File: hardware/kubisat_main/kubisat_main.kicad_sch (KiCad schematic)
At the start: 51 parts, among them J1 DEBUG_SWD, J2 Micro_SD_Card_Det1, J3 UART0, J4 POWER_IN, J5 IPX, Q1 BSS138, Q2 BSS138, SW1 BOOTSEL, SW2 RESET, U1 W25Q16JVSS, U2 RP2040, U3 NEO-6M-GPS, U4 XL1278-SMT, Y1 12MHz

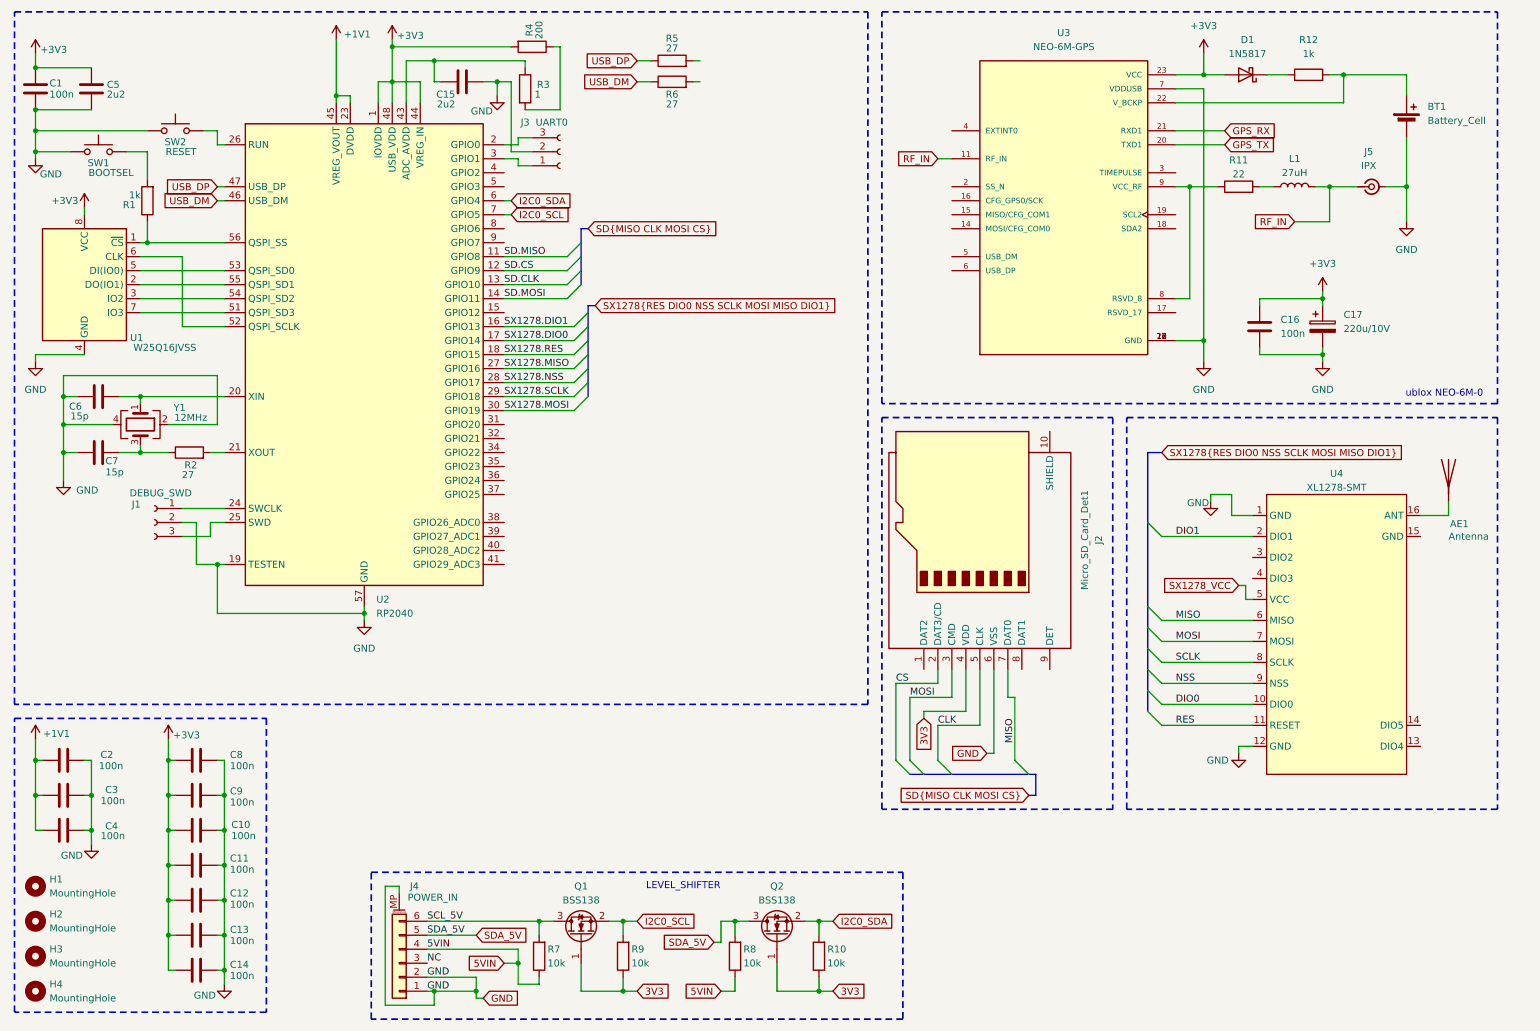
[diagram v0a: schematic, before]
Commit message: completed (?) mainboard schematic
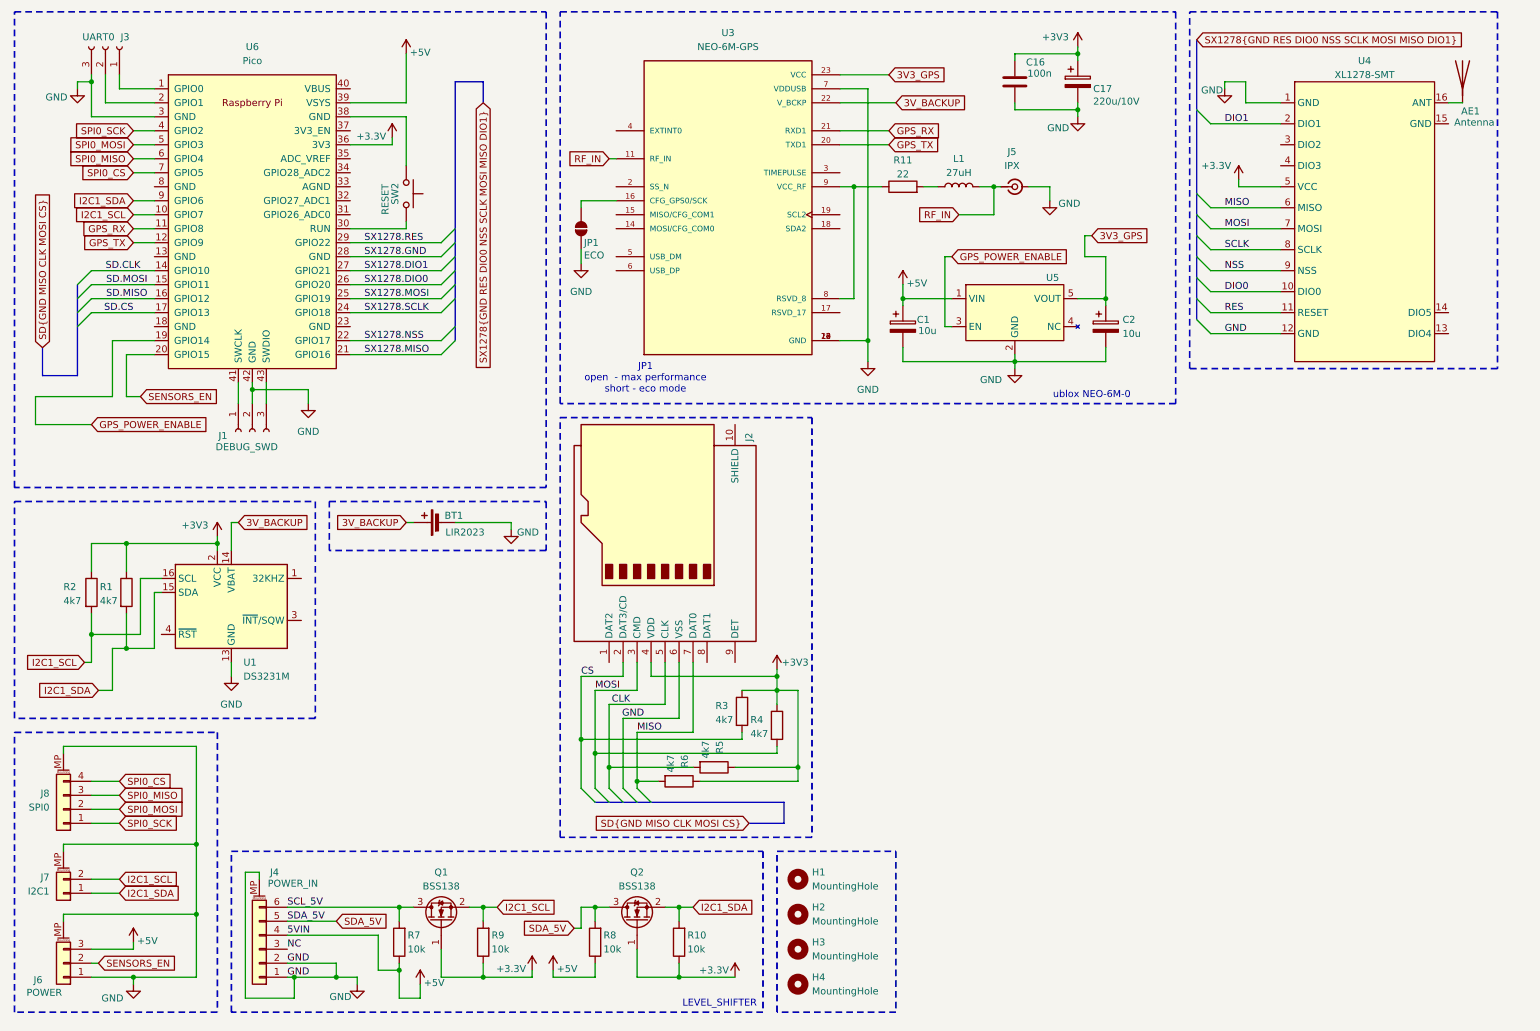
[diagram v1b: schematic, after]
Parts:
- removed C1, C10, C11, C12, C13, C14, C2, C3, C4, C8, C9: 100n, Capacitor_SMD:C_0805_2012Metric, symbol Device:C
- removed C15, C5: 2u2, Capacitor_SMD:C_0805_2012Metric, symbol Device:C
- removed C6, C7: 15p, Capacitor_SMD:C_0805_2012Metric, symbol Device:C
- removed D1: 1N5817, Diode_SMD:D_SOD-123, symbol Device:D_Schottky
- removed R12: 1k, Resistor_SMD:R_0805_2012Metric, symbol Device:R
- removed SW1: BOOTSEL, Button_Switch_SMD:SW_MEC_5GSH9, symbol Switch:SW_Push
- removed U1: W25Q16JVSS, Package_SO:SOIC-8_5.23x5.23mm_P1.27mm, symbol Memory_Flash:W25Q16JVSS
- removed U2: RP2040, Package_DFN_QFN:QFN-56-1EP_7x7mm_P0.4mm_EP3.2x3.2mm, symbol MCU_RaspberryPi:RP2040
- removed Y1: 12MHz, Crystal:Crystal_SMD_3225-4Pin_3.2x2.5mm, symbol Device:Crystal_GND24
- added C1, C2: 10u, Capacitor_Tantalum_SMD:CP_EIA-3216-18_Kemet-A, symbol Device:C_Polarized
- added J6: POWER, Connector_JST:JST_PH_B3B-PH-SM4-TB_1x03-1MP_P2.00mm_Vertical, symbol Connector_Generic_MountingPin:Conn_01x03_MountingPin
- added J7: I2C1, Connector_JST:JST_PH_B2B-PH-SM4-TB_1x02-1MP_P2.00mm_Vertical, symbol Connector_Generic_MountingPin:Conn_01x02_MountingPin
- added J8: SPI0, Connector_JST:JST_PH_B4B-PH-SM4-TB_1x04-1MP_P2.00mm_Vertical, symbol Connector_Generic_MountingPin:Conn_01x04_MountingPin
- added JP1: ECO, Jumper:SolderJumper-2_P1.3mm_Open_RoundedPad1.0x1.5mm, symbol Jumper:SolderJumper_2_Open
- added U1: DS3231M, Package_SO:SOIC-16W_7.5x10.3mm_P1.27mm, symbol Timer_RTC:DS3231M
- added U5: ~, Package_TO_SOT_SMD:SOT-23-5, symbol kubisat1:LDI8119-3.3EN
- added U6: Pico, KiCadLibraries:RPi_Pico_SMD_TH, symbol MCU_RaspberryPi_and_Boards:Pico
- BT1: value Battery_Cell -> LIR2023; footprint Battery:BatteryHolder_Seiko_MS621F -> Battery:BatteryHolder_Keystone_106_1x20mm
- J2: footprint Connector_Card:MR01A-01211 -> Connector_Card:J_SD_Card-micro_socket_A
- R1: value 1k -> 4k7; footprint (none) -> Resistor_SMD:R_0805_2012Metric
- R10, R7, R8, R9: footprint (none) -> Resistor_SMD:R_0805_2012Metric
- R2, R5, R6: value 27 -> 4k7; footprint (none) -> Resistor_SMD:R_0805_2012Metric
- R3: value 1 -> 4k7; footprint (none) -> Resistor_SMD:R_0805_2012Metric
- R4: value 200 -> 4k7; footprint (none) -> Resistor_SMD:R_0805_2012Metric
- SW2: footprint Button_Switch_SMD:SW_MEC_5GSH9 -> Button_Switch_SMD:SW_SPST_B3SL-1002P
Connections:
- net I2C0_SCL is gone; now on net I2C1_SCL: Q1.2 (S), R9.2
- net I2C0_SDA is gone; now on net I2C1_SDA: Q2.2 (S), R10.2
- net SX1278_VCC is gone; now on net +3.3V: U4.5 (VCC)
- net USB_DM is gone; now on net +3V3: R6.1
- net USB_DP is gone; now on net +3V3: R5.1
- net +3V3: now also J2.4 (VDD), R1.1, R2.1, R3.1, R4.1, U1.2 (VCC); no longer R4.2, U3.23 (VCC)
- net CLK: now also R5.2
- net CS: now also R3.2
- net GND: now also J3.3 (Pin_3), C1.2, C2.2, J6.1 (Pin_1), J6.MP (MountPin), J7.MP (MountPin), J8.MP (MountPin), JP1.2 (B), U1.10 (GND), U1.11 (GND), U1.12 (GND), U1.13 (GND), U1.5 (GND), U1.6 (GND), U1.7 (GND), U1.8 (GND), U1.9 (GND), U5.2 (GND), U6.3 (GND), U6.42 (GND); no longer J3.2 (Pin_2), SW2.1
- net GPS_RX: now also U6.11 (GPIO8)
- net GPS_TX: now also U6.12 (GPIO9)
- net MISO: now also R6.2
- net MOSI: now also R4.2
- net SD.CLK: now also U6.14 (GPIO10)
- net SD.CS: now also U6.17 (GPIO13)
- net SD.MISO: now also U6.16 (GPIO12)
- net SD.MOSI: now also U6.15 (GPIO11)
- net SX1278.DIO0: now also U6.26 (GPIO20)
- net SX1278.DIO1: now also U6.27 (GPIO21)
- net SX1278.MISO: now also U6.21 (GPIO16)
- net SX1278.MOSI: now also U6.25 (GPIO19)
- net SX1278.NSS: now also U6.22 (GPIO17)
- net SX1278.RES: now also U6.29 (GPIO22)
- net SX1278.SCLK: now also U6.24 (GPIO18)
- net I2C1_SCL: now reaches R2.2
- net I2C1_SCL: now also J7.2 (Pin_2), U1.16 (SCL), U6.10 (GPIO7)
- net 3V_BACKUP: now reaches BT1.1 (+), U3.22 (V_BCKP)
- net 3V_BACKUP: now also U1.14 (VBAT)
- net at SW2.2: now also U6.30 (RUN)
- net at J1.1 (Pin_1): now also U6.41 (SWCLK)
- net at J1.3 (Pin_3): now also U6.43 (SWDIO)
- net at J3.1 (Pin_1): now also U6.1 (GPIO0)
- net I2C1_SDA: now reaches R1.2
- net I2C1_SDA: now also J7.1 (Pin_1), U1.15 (SDA), U6.9 (GPIO6)
- net at U3.16 (CFG_GPS0/SCK): now also JP1.1 (A)
- net 3V3 renamed +3.3V
- net +3.3V: now also U6.36 (3V3); no longer J2.4 (VDD)
- net 5VIN renamed +5V
- net +5V: now also C1.1, J6.3 (Pin_3), U5.1 (VIN), U6.39 (VSYS)
- new net: SW2.1, U6.38 (GND)
- new net: J3.2 (Pin_2), U6.2 (GPIO1)
- new net 3V3_GPS: C2.1, U3.23 (VCC), U5.5 (VOUT)
- new net GPS_POWER_ENABLE: U5.3 (EN), U6.19 (GPIO14)
- new net SENSORS_EN: J6.2 (Pin_2), U6.20 (GPIO15)
- new net SPI0_CS: J8.4 (Pin_4), U6.7 (GPIO5)
- new net SPI0_MISO: J8.3 (Pin_3), U6.6 (GPIO4)
- new net SPI0_MOSI: J8.2 (Pin_2), U6.5 (GPIO3)
- new net SPI0_SCK: J8.1 (Pin_1), U6.4 (GPIO2)
- new net SX1278.GND: U6.28 (GND)
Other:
- note added: "JP1 open - max performance short - eco mode"
- moved on the sheet: AE1, C16, C17, H1, H2, H3, H4, J1, J2, J3, J4, J5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
